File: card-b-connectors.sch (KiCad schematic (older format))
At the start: 10 parts, among them J1 PCIe_x1, J2 AVR-ISP-6, J3 Conn_01x06, J4 Conn_01x01_Female, J5 Conn_01x01_Female

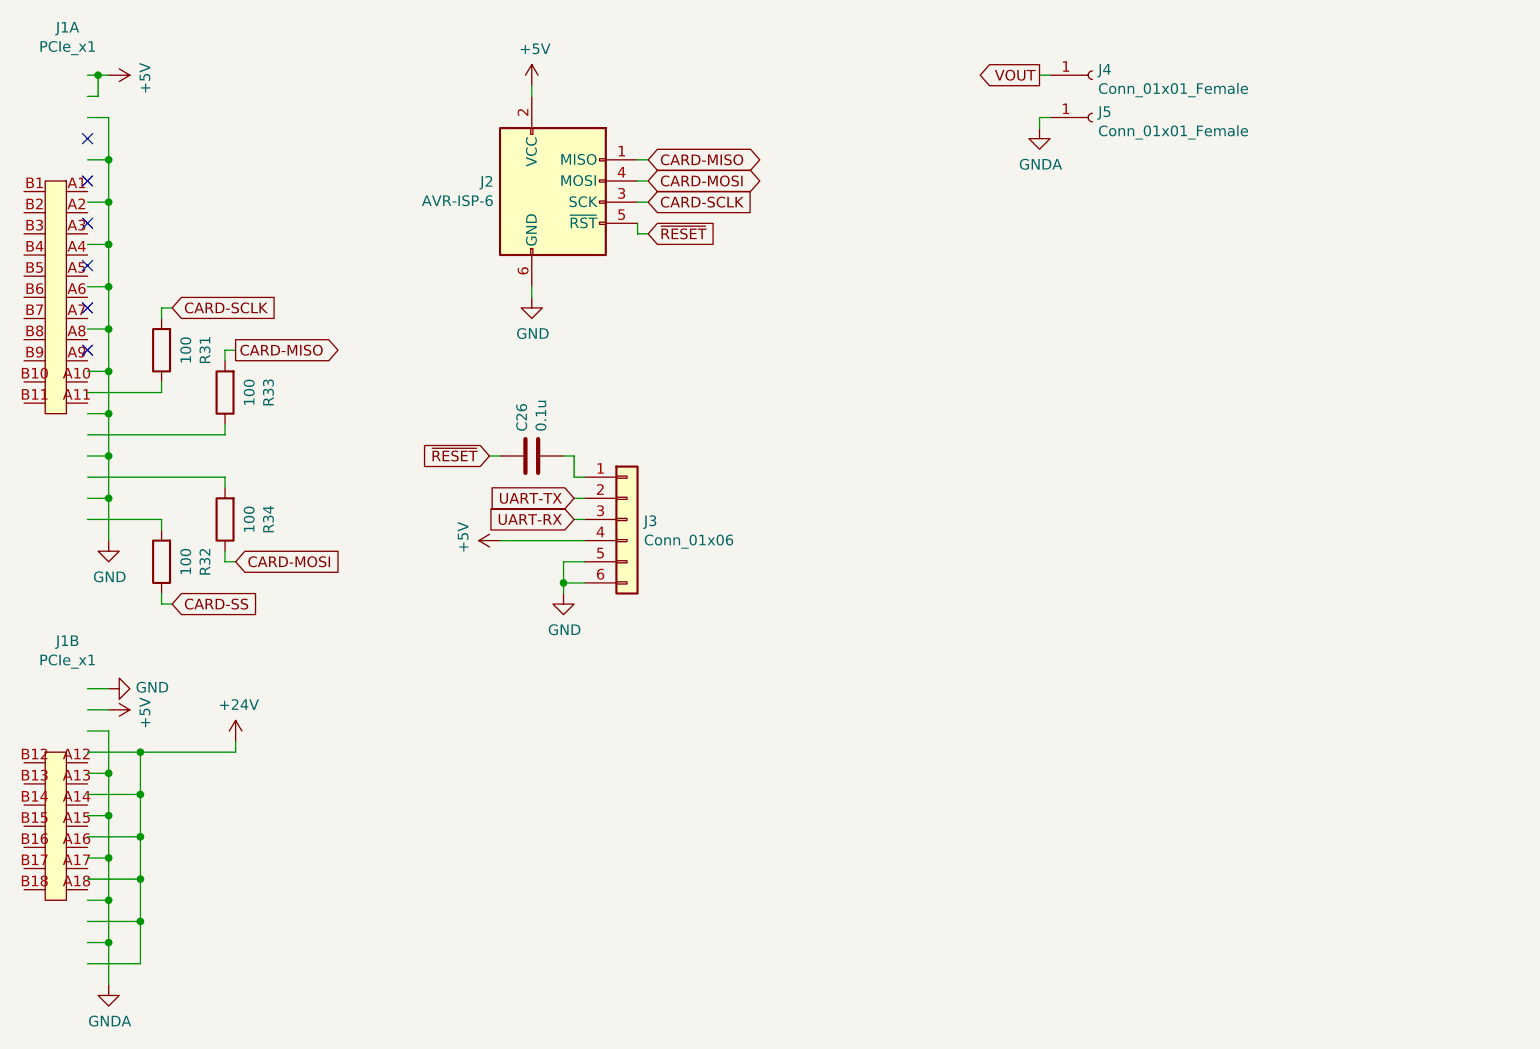
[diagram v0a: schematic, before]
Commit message: Update with notes and pending changes
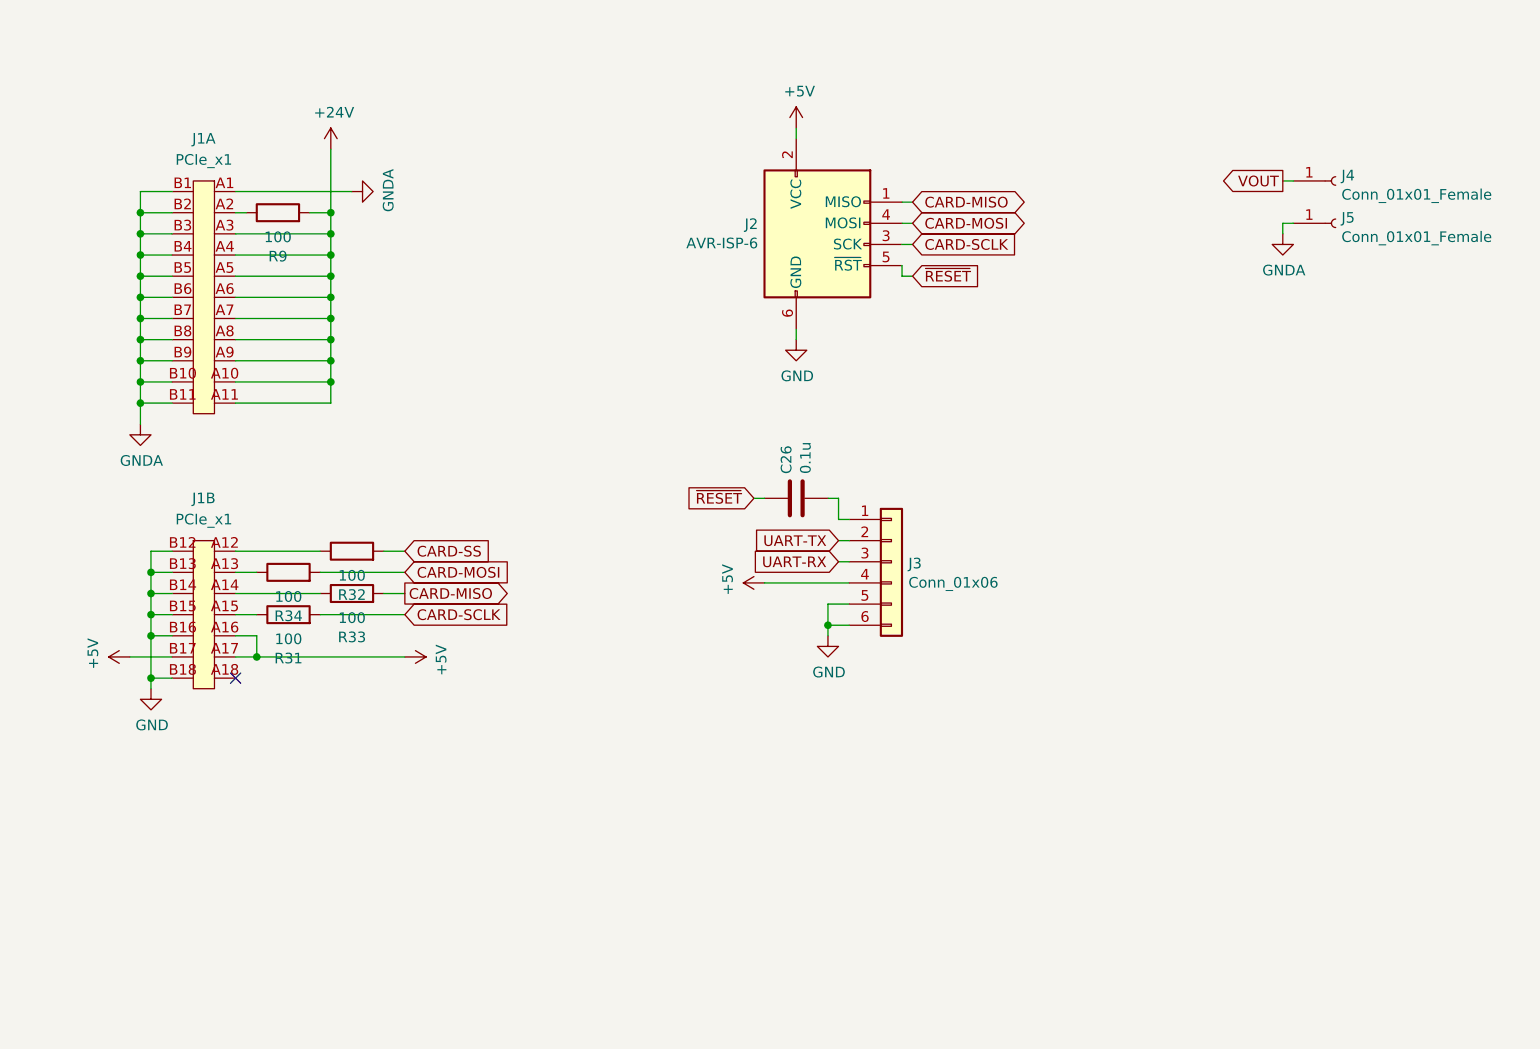
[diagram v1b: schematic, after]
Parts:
- added R9: 100, Resistor_SMD:R_0603_1608Metric_Pad1.05x0.95mm_HandSolder, symbol Device:R
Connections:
- wire segments 88 -> 90
- no-connect marks 6 -> 1
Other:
- moved on the sheet: C26, J1A, J1B, J2, J3, J4, J5, R31, R32, R33, R34
